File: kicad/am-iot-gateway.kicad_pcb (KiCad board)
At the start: 4 copper layers, 22 x 42 mm, 42 parts, among them J1 Bus_M.2_Socket_E, J3 GNSS Antenna, J4 RF Antenna, J5 NSIM-5-B, Q1 SS8050, Q2 SS8050, Q3 SS8050, U2 SIM7080G, U3 TXB0108RGY

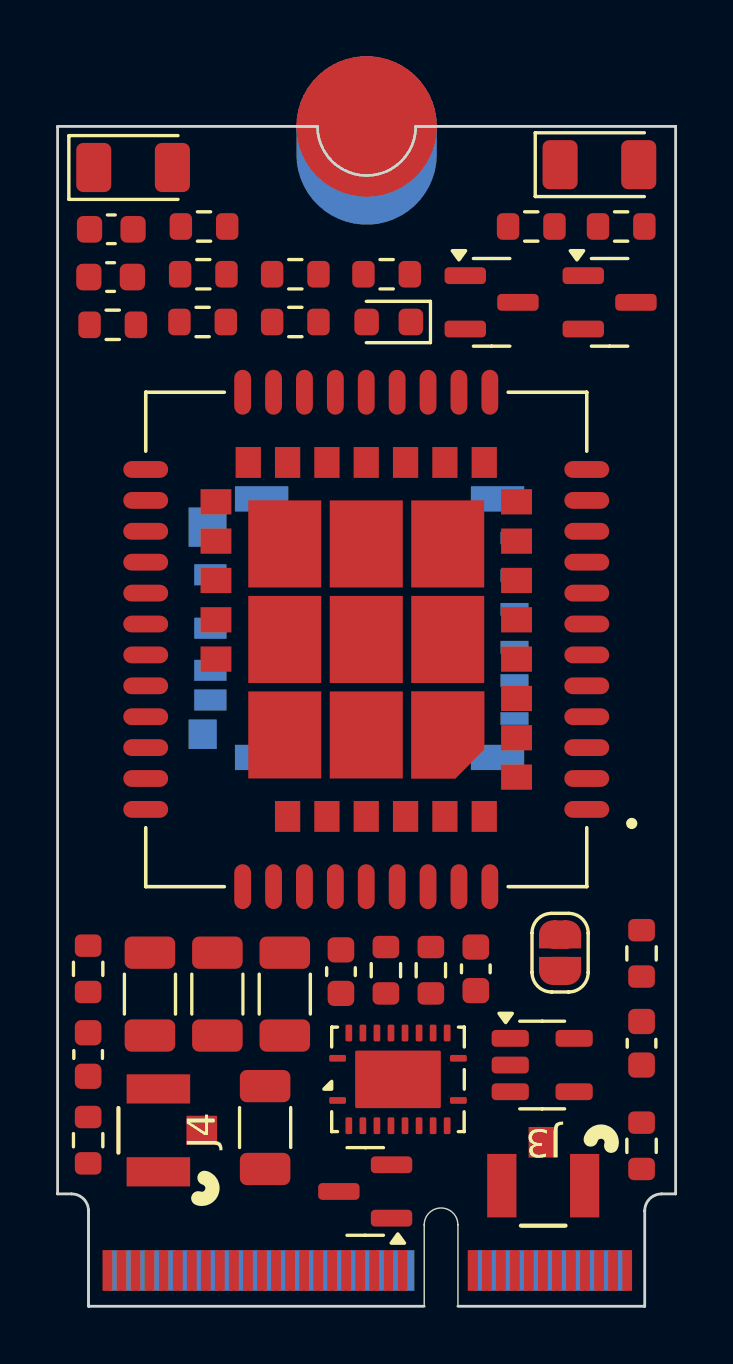
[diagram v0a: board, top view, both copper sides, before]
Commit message: Route PCB
Signed-off-by: JeffMboya <jangina.mboya@gmail.com>
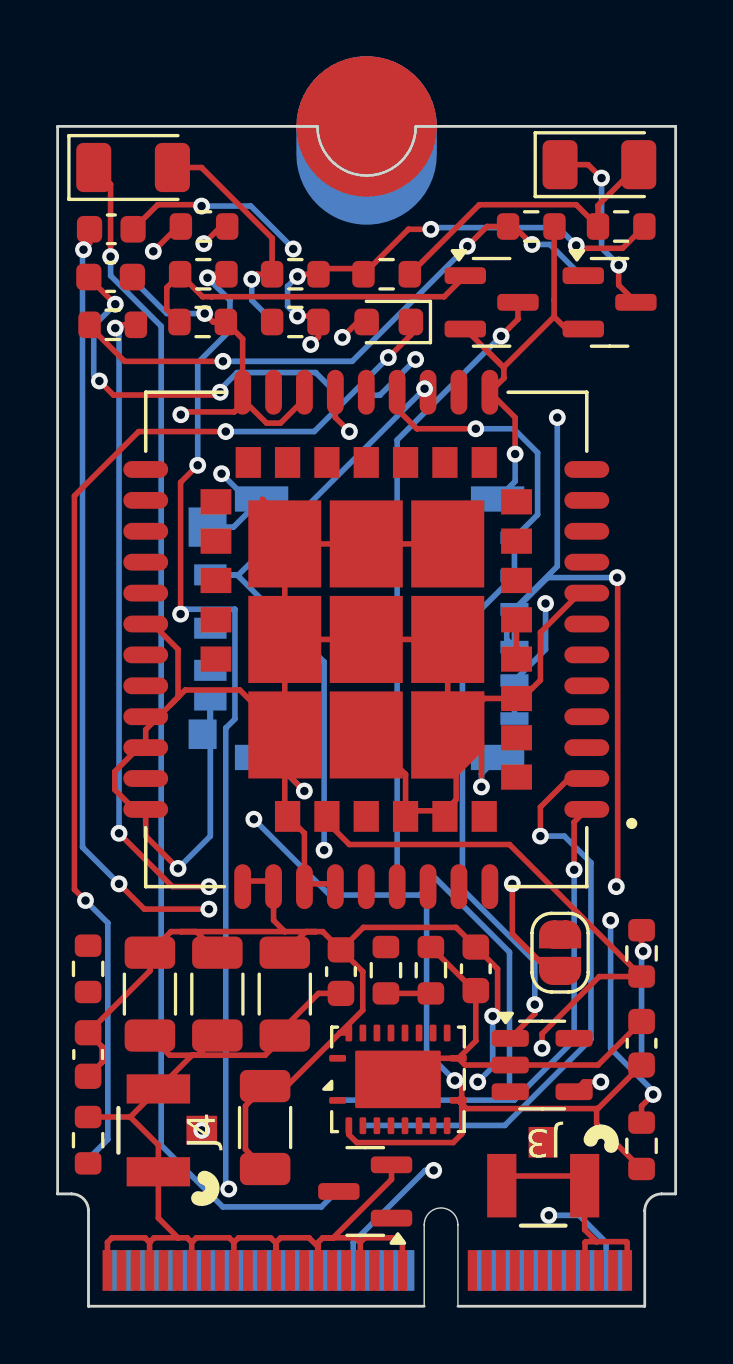
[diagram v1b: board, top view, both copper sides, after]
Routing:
- net GND: track 0.00 -> 185.8 mm, vias 0 -> 7
- net +1V8: track 0.00 -> 79.9 mm, vias 0 -> 8
- net +3V3: track 0.00 -> 72.3 mm, vias 0 -> 4
- net SIM7080G_PWR: track 0.00 -> 49.0 mm, vias 0 -> 4
- net Net-(D2-K): track 0.00 -> 43.3 mm, vias 0 -> 1
- net Net-(C7-Pad2): track 0.00 -> 42.7 mm, vias 0 -> 3
- net SIM_RST: track 0.00 -> 42.2 mm, vias 0 -> 5
- net Net-(D1-K): track 0.00 -> 39.3 mm, vias 0 -> 3
- net SIM_DATA: track 0.00 -> 34.7 mm, vias 0 -> 2
- net Net-(J4-Pad1): track 0.00 -> 33.9 mm, vias 0 -> 2
- net STATUS: track 0.00 -> 32.9 mm, vias 0 -> 3
- net SIM7080G_SDA: track 0.00 -> 31.6 mm, vias 0 -> 2
- net GNSS_ANT: track 0.00 -> 29.9 mm, vias 0 -> 2
- net Net-(JP1-B): track 0.00 -> 29.8 mm, vias 0 -> 1
- net SIM_CLK: track 0.00 -> 29.6 mm, vias 0 -> 2
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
